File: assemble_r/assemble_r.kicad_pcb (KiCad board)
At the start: 2 copper layers, 45 parts, among them J23 Conn_01x02_Pin, SW23 SW_Push, SW24 SW_Push, SW25 SW_Push, SW26 SW_Push, SW27 SW_Push, SW28 SW_Push, SW29 SW_Push, SW30 SW_Push, SW31 SW_Push, SW32 SW_Push, SW33 SW_Push, SW34 SW_Push, SW35 SW_Push, SW36 SW_Push, SW37 SW_Push, SW38 SW_Push, SW39 SW_Push, SW40 SW_Push, SW41 SW_Push, SW42 SW_Push, SW43 SW_Push, SW44 SW_Push, U23 Micon_BLEMicroPro

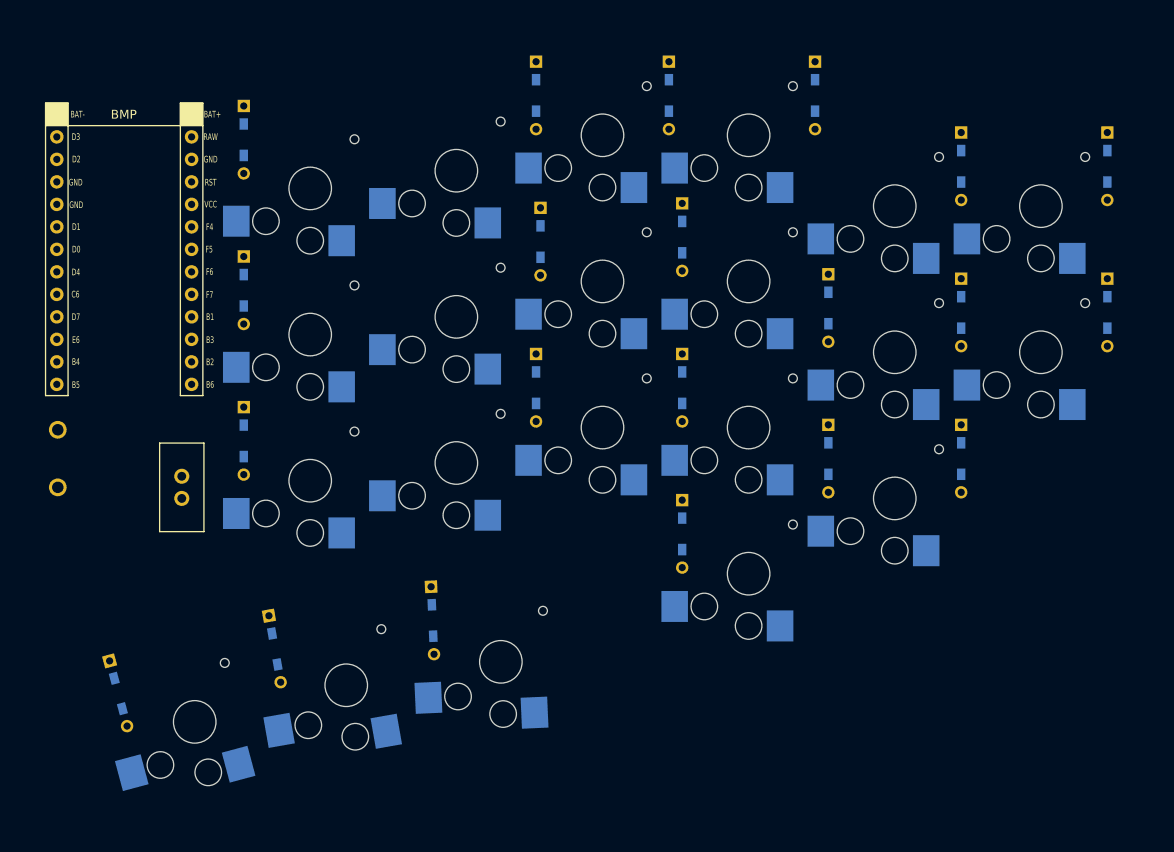
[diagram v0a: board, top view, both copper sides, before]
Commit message: feat: add outline
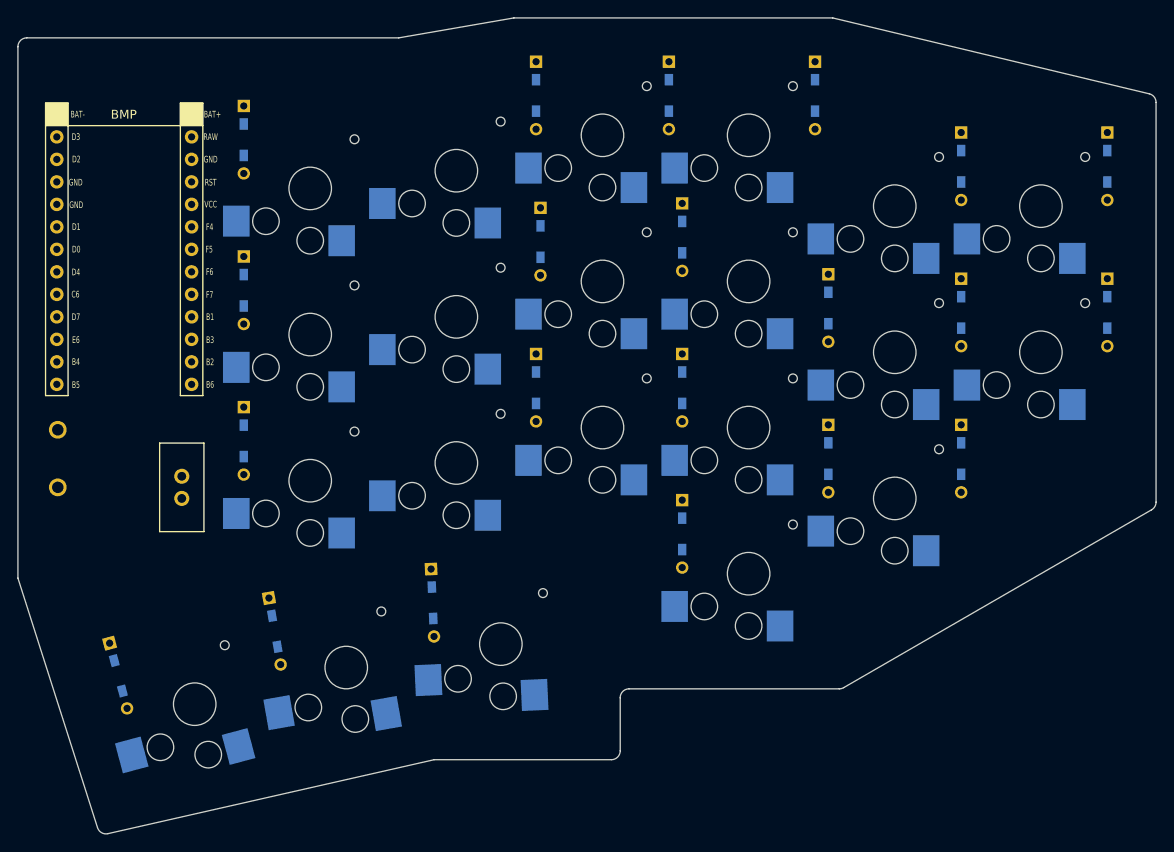
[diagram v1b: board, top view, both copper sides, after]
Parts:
- moved D26 2.00 mm to (49.3, 104.0)
- moved D30 2.00 mm to (67.0, 99.0)
- moved D34 2.00 mm to (84.8, 95.8)
- moved SW26 2.00 mm to (58.0, 107.2)
- moved SW30 2.00 mm to (75.1, 103.1)
- moved SW34 2.00 mm to (92.5, 100.4)
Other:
- board outline added: 128.5 x 92.1 mm
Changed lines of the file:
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@@
 	(footprint "kbd_SW:Choc_v2_Hotswap_1u_16.5"
 		(layer "F.Cu")
-		(at 57.95969 109.229467 15)
+		(at 57.95969 107.229467 15)
 		(property "Reference" "SW26"
 			(at -5.08 -6.35 15)
@@
 	(footprint "kbd_Parts:Diode_TH_SMD"
 		(layer "F.Cu")
-		(at 84.814316 97.781712 -87.5)
+		(at 84.814316 95.781712 -87.5)
 		(descr "Resitance 3 pas")
 		(tags "R")
@@
 	(footprint "kbd_Parts:Diode_TH_SMD"
 		(layer "F.Cu")
-		(at 49.337035 106.027055 -75)
+		(at 49.337035 104.027055 -75)
 		(descr "Resitance 3 pas")
 		(tags "R")
@@
 	(footprint "kbd_SW:Choc_v2_Hotswap_1u_16.5"
 		(layer "F.Cu")
-		(at 75.06811 105.095004 10)
+		(at 75.06811 103.095004 10)
 		(property "Reference" "SW30"
 			(at -5.08 -6.349999 10)
@@
 		)
 		(fp_line
-			(start -0.850002 8.2)
+			(start -0.850003 8.2)
 			(end -0.85 3.6)
 			(stroke
@@
 	(footprint "kbd_Parts:Diode_TH_SMD"
 		(layer "F.Cu")
-		(at 67 101 -80)
+		(at 67 99 -80)
 		(descr "Resitance 3 pas")
 		(tags "R")
@@
 		)
 		(pad "1" thru_hole rect
-			(at -3.810002 0 280)
+			(at -3.810003 0 280)
 			(size 1.397 1.397)
 			(drill 0.8128)
@@
 		)
 		(pad "2" thru_hole circle
-			(at 3.810002 0 280)
+			(at 3.810003 0 280)
 			(size 1.397 1.397)
 			(drill 0.8128)
@@
 	(footprint "kbd_SW:Choc_v2_Hotswap_1u_16.5"
 		(layer "F.Cu")
-		(at 92.525274 102.449808 2.5)
+		(at 92.525274 100.449808 2.5)
 		(property "Reference" "SW34"
 			(at -5.08 -6.35 2.5)
@@
 		)
 		(fp_line
-			(start -4.6 6.000002)
+			(start -4.6 6.000003)
 			(end -4.6 1.4)
 			(stroke
@@
 		)
 		(fp_line
-			(start -1.3 7.989998)
+			(start -1.3 7.989997)
 			(end -1.3 3.6)
 			(stroke
@@
 		(fp_line
 			(start -0.4 8.2)
-			(end -0.399998 3.6)
+			(end -0.399997 3.6)
 			(stroke
 				(width 0.15)
@@
 		)
 		(pad "" np_thru_hole circle
-			(at 5.000002 -5.55 2.5)
+			(at 5.000003 -5.55 2.5)
 			(size 1 1)
 			(drill oval 1)
@@
 		(embedded_fonts no)
 	)
+	(gr_arc
+		(start 48.161805 121.849991)
+		(mid 47.434731 121.73721)
+		(end 46.981573 121.15755)
+		(stroke
+			(width 0.05)
+			(type default)
+		)
+		(layer "Edge.Cuts")
+	)
+	(gr_line
+		(start 107 105.5)
+		(end 130.731933 105.5)
+		(stroke
+			(width 0.05)
+			(type default)
+		)
+		(layer "Edge.Cuts")
+	)
+	(gr_line
+		(start 85 113.5)
+		(end 105 113.5)
+		(stroke
+			(width 0.05)
+			(type default)
+		)
+		(layer "Edge.Cuts")
+	)
+	(gr_line
+		(start 94 29.75)
+		(end 130 29.75)
+		(stroke
+			(width 0.05)
+			(type default)
+		)
+		(layer "Edge.Cuts")
+	)
+	(gr_line
+		(start 131.232123 105.365916)
+		(end 165.992057 85.287098)
+		(stroke
+			(width 0.05)
+			(type default)
+		)
+		(layer "Edge.Cuts")
+	)
+	(gr_arc
+		(start 131.232123 105.365916)
+		(mid 130.990856 105.465889)
+		(end 130.731933 105.5)
+		(stroke
+			(width 0.05)
+			(type default)
+		)
+		(layer "Edge.Cuts")
+	)
+	(gr_arc
+		(start 106 112.5)
+		(mid 105.707107 113.207107)
+		(end 105 113.5)
+		(stroke
+			(width 0.05)
+			(type default)
+		)
+		(layer "Edge.Cuts")
+	)
+	(gr_line
+		(start 37 32)
+		(end 37 32)
+		(stroke
+			(width 0.05)
+			(type default)
+		)
+		(layer "Edge.Cuts")
+	)
+	(gr_line
+		(start 48.161805 121.849991)
+		(end 85 113.5)
+		(stroke
+			(width 0.05)
+			(type default)
+		)
+		(layer "Edge.Cuts")
+	)
+	(gr_line
+		(start 130 29.75)
+		(end 165.733121 38.316159)
+		(stroke
+			(width 0.05)
+			(type default)
+		)
+		(layer "Edge.Cuts")
+	)
+	(gr_line
+		(start 38 93)
+		(end 46.981573 121.15755)
+		(stroke
+			(width 0.05)
+			(type default)
+		)
+		(layer "Edge.Cuts")
+	)
+	(gr_line
+		(start 128.5 29.5)
+		(end 128.5 29.5)
+		(stroke
+			(width 0.05)
+			(type default)
+		)
+		(layer "Edge.Cuts")
+	)
+	(gr_line
+		(start 94 29.75)
+		(end 81 32)
+		(stroke
+			(width 0.05)
+			(type default)
+		)
+		(layer "Edge.Cuts")
+	)
+	(gr_arc
+		(start 38 33)
+		(mid 38.292893 32.292889)
+		(end 39 32)
+		(stroke
+			(width 0.05)
+			(type default)
+		)
+		(layer "Edge.Cuts")
+	)
+	(gr_arc
+		(start 166.5 84.416535)
+		(mid 166.363729 84.920491)
+		(end 165.992057 85.287098)
+		(stroke
+			(width 0.05)
+			(type default)
+		)
+		(layer "Edge.Cuts")
+	)
+	(gr_line
+		(start 81 32)
+		(end 39 32)
+		(stroke
+			(width 0.05)
+			(type default)
+		)
+		(layer "Edge.Cuts")
+	)
+	(gr_line
+		(start 166.5 39.288607)
+		(end 166.5 84.416535)
+		(stroke
+			(width 0.05)
+			(type default)
+		)
+		(layer "Edge.Cuts")
+	)
+	(gr_arc
+		(start 106 106.5)
+		(mid 106.292893 105.792893)
+		(end 107 105.5)
+		(stroke
+			(width 0.05)
+			(type default)
+		)
+		(layer "Edge.Cuts")
+	)
+	(gr_line
+		(start 38 33)
+		(end 38 93)
+		(stroke
+			(width 0.05)
+			(type default)
+		)
+		(layer "Edge.Cuts")
+	)
+	(gr_arc
+		(start 165.733121 38.316159)
+		(mid 166.285217 38.669379)
+		(end 166.5 39.288607)
+		(stroke
+			(width 0.05)
+			(type default)
+		)
+		(layer "Edge.Cuts")
+	)
+	(gr_line
+		(start 106 112.5)
+		(end 106 106.5)
+		(stroke
+			(width 0.05)
+			(type default)
+		)
+		(layer "Edge.Cuts")
+	)
 	(embedded_fonts no)
